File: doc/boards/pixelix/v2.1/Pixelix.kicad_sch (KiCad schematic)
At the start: 28 parts, among them J1 Conn_01x02, J2 Conn_01x02, J3 Conn_01x03, J4 Conn_01x02, J5 Conn_02x05_Odd_Even, J7 Conn_01x03, J8 Conn_01x02, Q1 NMOS_GSD_BSS138, Q2 PMOS_GDS_STD26P3LLH6

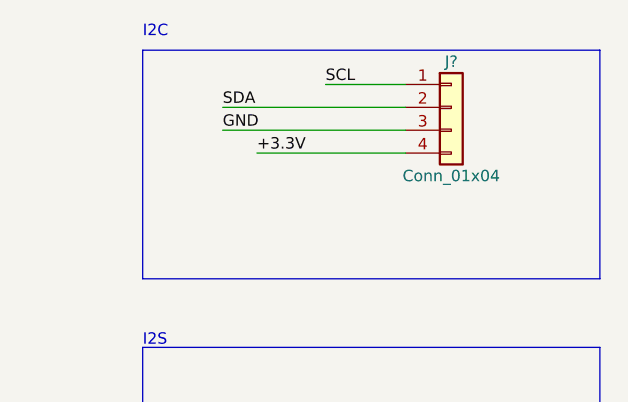
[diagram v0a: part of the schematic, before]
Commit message: 更新使用说明
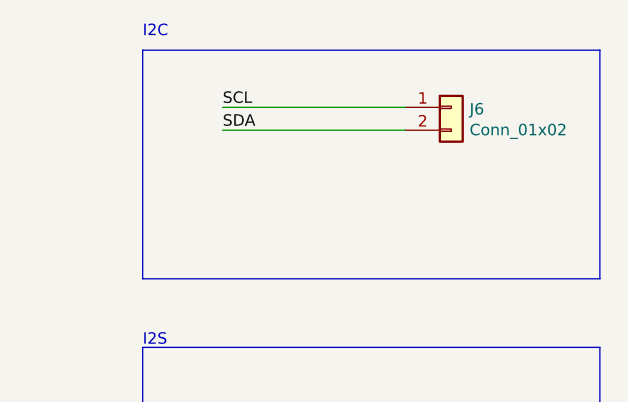
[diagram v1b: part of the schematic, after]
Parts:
- J6: renamed from J?; value Conn_01x04 -> Conn_01x02; footprint (none) -> footprints:66200211022; symbol Connector_Generic:Conn_01x04 -> Connector_Generic:Conn_01x02
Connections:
- net GND: no longer J6.3 (Pin_3)
- removed net +3.3V: J6.4 (Pin_4)
